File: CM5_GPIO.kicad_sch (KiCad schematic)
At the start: 30 parts, among them J11 RTC Battery Port, J12 RTC Battery Conn, J14 4x nano-fit, J3 2222, SW1 SW_Push, SW2 SW_Push

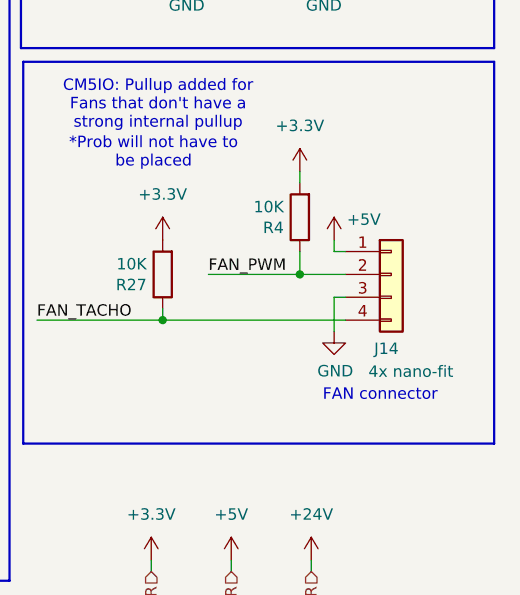
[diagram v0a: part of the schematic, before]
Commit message: chang
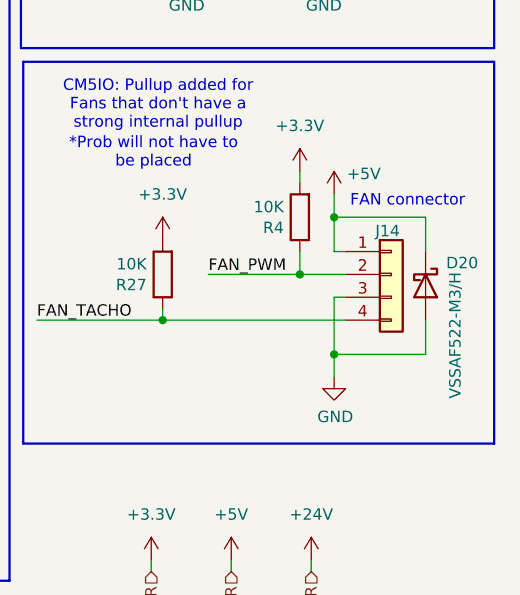
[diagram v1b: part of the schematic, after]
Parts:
- added D20: VSSAF522-M3/H, UTSVT_Passives:MMDL101T1G, symbol Diode:C3D25170H
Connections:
- net +5V: now also D20.1 (K)
- net GND: now also D20.2 (A)
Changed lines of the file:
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@@
 	(text "FAN connector\n"
 		(exclude_from_sim no)
-		(at 256.54 120.904 0)
+		(at 259.588 99.314 0)
 		(effects
 			(font
@@
 	)
 	(junction
+		(at 257.81 100.33)
+		(diameter 0)
+		(color 0 0 0 0)
+	)
+	(junction
 		(at 180.34 25.4)
 		(diameter 0)
@@
 	)
 	(junction
+		(at 257.81 115.57)
+		(diameter 0)
+		(color 0 0 0 0)
+	)
+	(junction
 		(at 43.18 72.39)
 		(diameter 0)
@@
 	(wire
 		(pts
+			(xy 267.97 100.33) (xy 257.81 100.33)
+		)
+		(stroke
+			(width 0)
+			(type default)
+		)
+	)
+	(wire
+		(pts
 			(xy 224.79 111.76) (xy 238.76 111.76)
 		)
@@
 	(wire
 		(pts
+			(xy 257.81 115.57) (xy 267.97 115.57)
+		)
+		(stroke
+			(width 0)
+			(type default)
+		)
+	)
+	(wire
+		(pts
 			(xy 119.38 148.59) (xy 105.41 148.59)
 		)
@@
 	(wire
 		(pts
-			(xy 257.81 104.14) (xy 257.81 102.87)
+			(xy 257.81 100.33) (xy 257.81 104.14)
 		)
 		(stroke
@@
 	(wire
 		(pts
+			(xy 257.81 97.79) (xy 257.81 100.33)
+		)
+		(stroke
+			(width 0)
+			(type default)
+		)
+	)
+	(wire
+		(pts
 			(xy 106.68 41.91) (xy 106.68 49.53)
 		)
@@
 	(wire
 		(pts
+			(xy 267.97 104.14) (xy 267.97 100.33)
+		)
+		(stroke
+			(width 0)
+			(type default)
+		)
+	)
+	(wire
+		(pts
 			(xy 255.27 48.26) (xy 266.7 48.26)
 		)
@@
 	(wire
 		(pts
+			(xy 267.97 115.57) (xy 267.97 111.76)
+		)
+		(stroke
+			(width 0)
+			(type default)
+		)
+	)
+	(wire
+		(pts
 			(xy 43.18 97.79) (xy 44.45 97.79)
 		)
@@
 	(wire
 		(pts
-			(xy 257.81 109.22) (xy 257.81 113.03)
+			(xy 257.81 109.22) (xy 257.81 115.57)
 		)
 		(stroke
@@
 	(wire
 		(pts
+			(xy 257.81 115.57) (xy 257.81 118.11)
+		)
+		(stroke
+			(width 0)
+			(type default)
+		)
+	)
+	(wire
+		(pts
 			(xy 43.18 115.57) (xy 43.18 125.73)
 		)
@@
 	(symbol
 		(lib_id "power:GND")
-		(at 257.81 113.03 0)
+		(at 257.81 118.11 0)
 		(unit 1)
 		(exclude_from_sim no)
@@
 		(dnp no)
 		(property "Reference" "#PWR037"
-			(at 257.81 119.38 0)
+			(at 257.81 124.46 0)
 			(effects
 				(font
@@
 		)
 		(property "Value" "GND"
-			(at 257.937 117.4242 0)
+			(at 257.937 122.5042 0)
 			(effects
 				(font
@@
 		)
 		(property "Footprint" ""
-			(at 257.81 113.03 0)
+			(at 257.81 118.11 0)
 			(effects
 				(font
@@
 		)
 		(property "Datasheet" ""
-			(at 257.81 113.03 0)
+			(at 257.81 118.11 0)
 			(effects
 				(font
@@
 		)
 		(property "Description" "Power symbol creates a global label with name \"GND\" , ground"
-			(at 257.81 113.03 0)
+			(at 257.81 118.11 0)
 			(effects
 				(font
@@
 		(dnp no)
 		(property "Reference" "J14"
-			(at 262.255 114.935 0)
+			(at 262.382 101.854 0)
 			(effects
 				(font
@@
 				)
 				(justify left)
+				(hide yes)
 			)
 		)
@@
 	(symbol
 		(lib_id "power:+12V")
-		(at 257.81 102.87 0)
+		(at 257.81 97.79 0)
 		(unit 1)
 		(exclude_from_sim no)
@@
 		(dnp no)
 		(property "Reference" "#PWR039"
-			(at 257.81 106.68 0)
+			(at 257.81 101.6 0)
 			(effects
 				(font
@@
 		)
 		(property "Value" "+5V"
-			(at 261.112 100.584 0)
+			(at 261.112 95.504 0)
 			(effects
 				(font
@@
 		)
 		(property "Footprint" ""
-			(at 257.81 102.87 0)
+			(at 257.81 97.79 0)
 			(effects
 				(font
@@
 		)
 		(property "Datasheet" ""
-			(at 257.81 102.87 0)
+			(at 257.81 97.79 0)
 			(effects
 				(font
@@
 		)
 		(property "Description" "Power symbol creates a global label with name \"+12V\""
-			(at 257.81 102.87 0)
+			(at 257.81 97.79 0)
 			(effects
 				(font
@@
 					(unit 1)
 				)
+			)
+		)
+	)
+	(symbol
+		(lib_id "Diode:C3D25170H")
+		(at 267.97 107.95 270)
+		(unit 1)
+		(exclude_from_sim no)
+		(in_bom yes)
+		(on_board yes)
+		(dnp no)
+		(property "Reference" "D20"
+			(at 270.256 105.41 90)
+			(effects
+				(font
+					(size 1.27 1.27)
+				)
+				(justify left)
+			)
+		)
+		(property "Value" "VSSAF522-M3/H"
+			(at 271.272 106.426 0)
+			(effects
+				(font
+					(size 1.27 1.27)
+				)
+				(justify left)
+			)
+		)
+		(property "Footprint" "UTSVT_Passives:MMDL101T1G"
+			(at 263.525 107.95 0)
+			(effects
+				(font
+					(size 1.27 1.27)
+				)
+				(hide yes)
+			)
+		)
+		(property "Datasheet" "https://www.mouser.com/ProductDetail/Vishay-General-Semiconductor/VSSAF522-M3-H?qs=UkDUCjYnTB00gpgD%2Fb%2Fw%252BA%3D%3D"
+			(at 267.97 107.95 0)
+			(effects
+				(font
+					(size 1.27 1.27)
+				)
+				(hide yes)
+			)
+		)
+		(property "Description" ""
+			(at 267.97 107.95 0)
+			(effects
+				(font
+					(size 1.27 1.27)
+				)
+				(hide yes)
+			)
+		)
+		(property "Manufactuerer" "Vishay General Semiconductor "
+			(at 267.97 107.95 90)
+			(effects
+				(font
+					(size 1.27 1.27)
+				)
+				(hide yes)
+			)
+		)
+		(property "P/N" "VSSAF522-M3/H"
+			(at 267.97 107.95 90)
+			(effects
+				(font
+					(size 1.27 1.27)
+				)
+				(hide yes)
+			)
+		)
+		(pin "1"
+		)
+		(pin "2"
+		)
+		(instances
+			(project "PiBoard"
+				(path "/e4d65698-b8ec-4bf6-9f2b-a5010377155a/353ee88d-a044-4c9d-80a8-948975426026"
+					(reference "D20")
+					(unit 1)
+				)
